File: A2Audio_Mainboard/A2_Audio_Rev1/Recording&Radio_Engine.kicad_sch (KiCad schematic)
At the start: 28 parts, among them IC1 ES9822QPRO, U11 SI4732-A10-GS, U12 OPA1612AIDR, U16 AP2112K-3.3, U17 AP2112K-1.8, Y1 Crystal

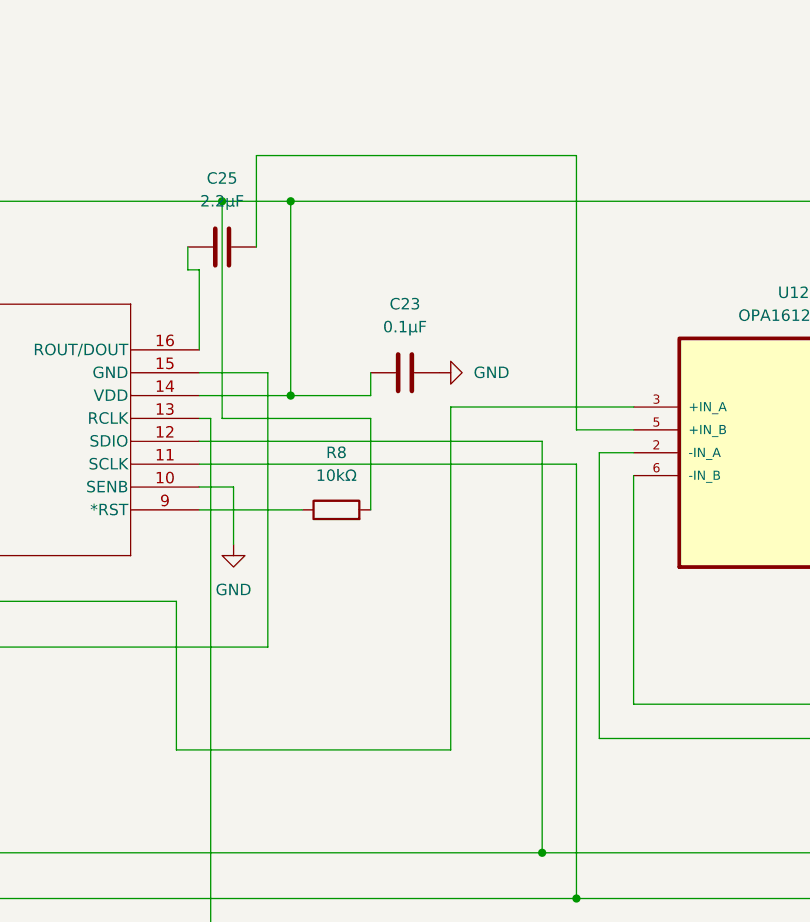
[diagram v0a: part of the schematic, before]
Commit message: More Refinement
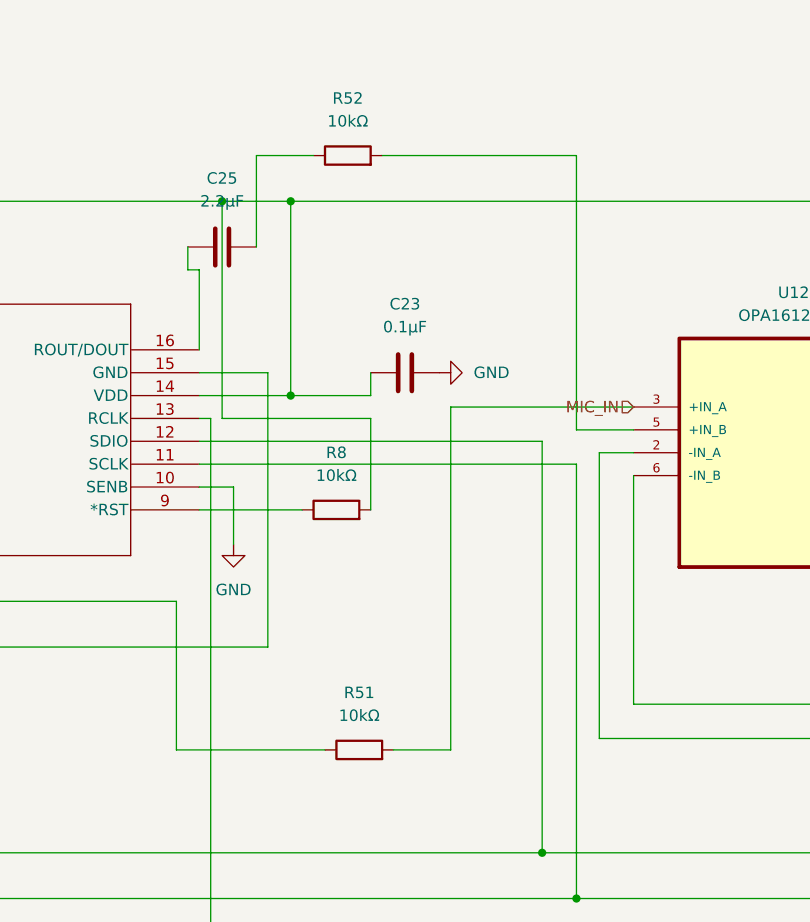
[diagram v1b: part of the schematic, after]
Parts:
- added R51, R52: 10kΩ, symbol symbols:R
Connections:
- net at C24.1: now also R51.1; no longer U12.3 (+IN_A)
- net at C25.2: now also R52.1; no longer U12.5 (+IN_B)
- new net: R52.2, U12.5 (+IN_B)
- new net MIC_IN: R51.2, U12.3 (+IN_A)
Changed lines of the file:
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@@
+	(wire
+		(pts
+			(xy 186.69 91.44) (xy 193.04 91.44)
+		)
+		(stroke
+			(width 0)
+			(type default)
+		)
+	)
 	(wire
 		(pts
@@
 	(wire
 		(pts
+			(xy 185.42 25.4) (xy 207.01 25.4)
+		)
+		(stroke
+			(width 0)
+			(type default)
+		)
+	)
+	(wire
+		(pts
 			(xy 318.77 29.21) (xy 318.77 21.59)
 		)
@@
 	(wire
 		(pts
-			(xy 171.45 25.4) (xy 207.01 25.4)
+			(xy 171.45 25.4) (xy 177.8 25.4)
 		)
 		(stroke
@@
 	(wire
 		(pts
-			(xy 162.56 91.44) (xy 193.04 91.44)
+			(xy 162.56 91.44) (xy 179.07 91.44)
 		)
 		(stroke
@@
 			)
 			(justify left)
+		)
+	)
+	(hierarchical_label "MIC_IN"
+		(shape input)
+		(at 213.36 53.34 180)
+		(effects
+			(font
+				(size 1.27 1.27)
+			)
+			(justify right)
 		)
 	)
@@
 	)
 	(symbol
+		(lib_id "symbols:R")
+		(at 182.88 91.44 90)
+		(unit 1)
+		(body_style 1)
+		(exclude_from_sim no)
+		(in_bom yes)
+		(on_board yes)
+		(in_pos_files yes)
+		(dnp no)
+		(fields_autoplaced yes)
+		(property "Reference" "R51"
+			(at 182.88 85.09 90)
+			(show_name no)
+			(do_not_autoplace no)
+			(effects
+				(font
+					(size 1.27 1.27)
+				)
+			)
+		)
+		(property "Value" "10kΩ"
+			(at 182.88 87.63 90)
+			(show_name no)
+			(do_not_autoplace no)
+			(effects
+				(font
+					(size 1.27 1.27)
+				)
+			)
+		)
+		(property "Footprint" ""
+			(at 182.88 93.218 90)
+			(hide yes)
+			(show_name no)
+			(do_not_autoplace no)
+			(effects
+				(font
+					(size 1.27 1.27)
+				)
+			)
+		)
+		(property "Datasheet" ""
+			(at 182.88 91.44 0)
+			(hide yes)
+			(show_name no)
+			(do_not_autoplace no)
+			(effects
+				(font
+					(size 1.27 1.27)
+				)
+			)
+		)
+		(property "Description" "Resistor"
+			(at 182.88 91.44 0)
+			(hide yes)
+			(show_name no)
+			(do_not_autoplace no)
+			(effects
+				(font
+					(size 1.27 1.27)
+				)
+			)
+		)
+		(pin "2"
+		)
+		(pin "1"
+		)
+		(instances
+			(project "A2_Audio_Rev1"
+				(path "/6bc02254-56bf-4f9a-8c1a-77c700c92092/a9d53889-2e3e-474f-9b5d-b71fef7f778c"
+					(reference "R51")
+					(unit 1)
+				)
+			)
+		)
+	)
+	(symbol
 		(lib_id "symbols:C")
 		(at 264.16 44.45 0)
@@
 					(unit 1)
 				)
+			)
+		)
+	)
+	(symbol
+		(lib_id "symbols:R")
+		(at 181.61 25.4 90)
+		(unit 1)
+		(body_style 1)
+		(exclude_from_sim no)
+		(in_bom yes)
+		(on_board yes)
+		(in_pos_files yes)
+		(dnp no)
+		(fields_autoplaced yes)
+		(property "Reference" "R52"
+			(at 181.61 19.05 90)
+			(show_name no)
+			(do_not_autoplace no)
+			(effects
+				(font
+					(size 1.27 1.27)
+				)
+			)
+		)
+		(property "Value" "10kΩ"
+			(at 181.61 21.59 90)
+			(show_name no)
+			(do_not_autoplace no)
+			(effects
+				(font
+					(size 1.27 1.27)
+				)
+			)
+		)
+		(property "Footprint" ""
+			(at 181.61 27.178 90)
+			(hide yes)
+			(show_name no)
+			(do_not_autoplace no)
+			(effects
+				(font
+					(size 1.27 1.27)
+				)
+			)
+		)
+		(property "Datasheet" ""
+			(at 181.61 25.4 0)
+			(hide yes)
+			(show_name no)
+			(do_not_autoplace no)
+			(effects
+				(font
+					(size 1.27 1.27)
+				)
+			)
+		)
+		(property "Description" "Resistor"
+			(at 181.61 25.4 0)
+			(hide yes)
+			(show_name no)
+			(do_not_autoplace no)
+			(effects
+				(font
+					(size 1.27 1.27)
+				)
+			)
+		)
+		(pin "2"
+		)
+		(pin "1"
+		)
+		(instances
+			(project "A2_Audio_Rev1"
+				(path "/6bc02254-56bf-4f9a-8c1a-77c700c92092/a9d53889-2e3e-474f-9b5d-b71fef7f778c"
+					(reference "R52")
+					(unit 1)
+				)
